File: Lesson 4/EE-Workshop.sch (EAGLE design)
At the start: 1 part

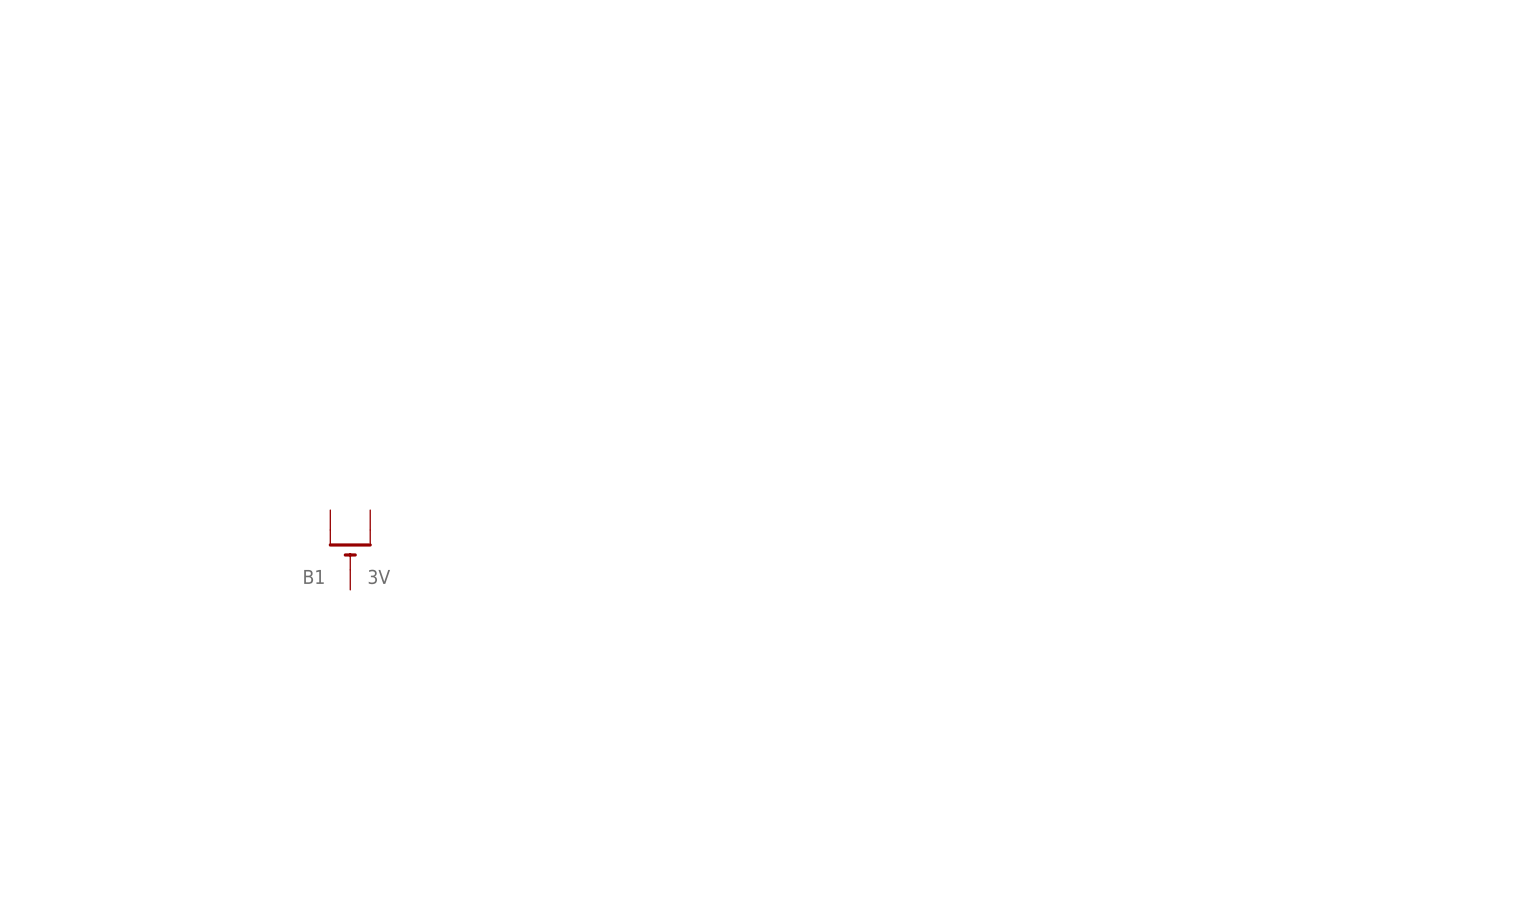
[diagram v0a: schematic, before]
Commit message: Piano
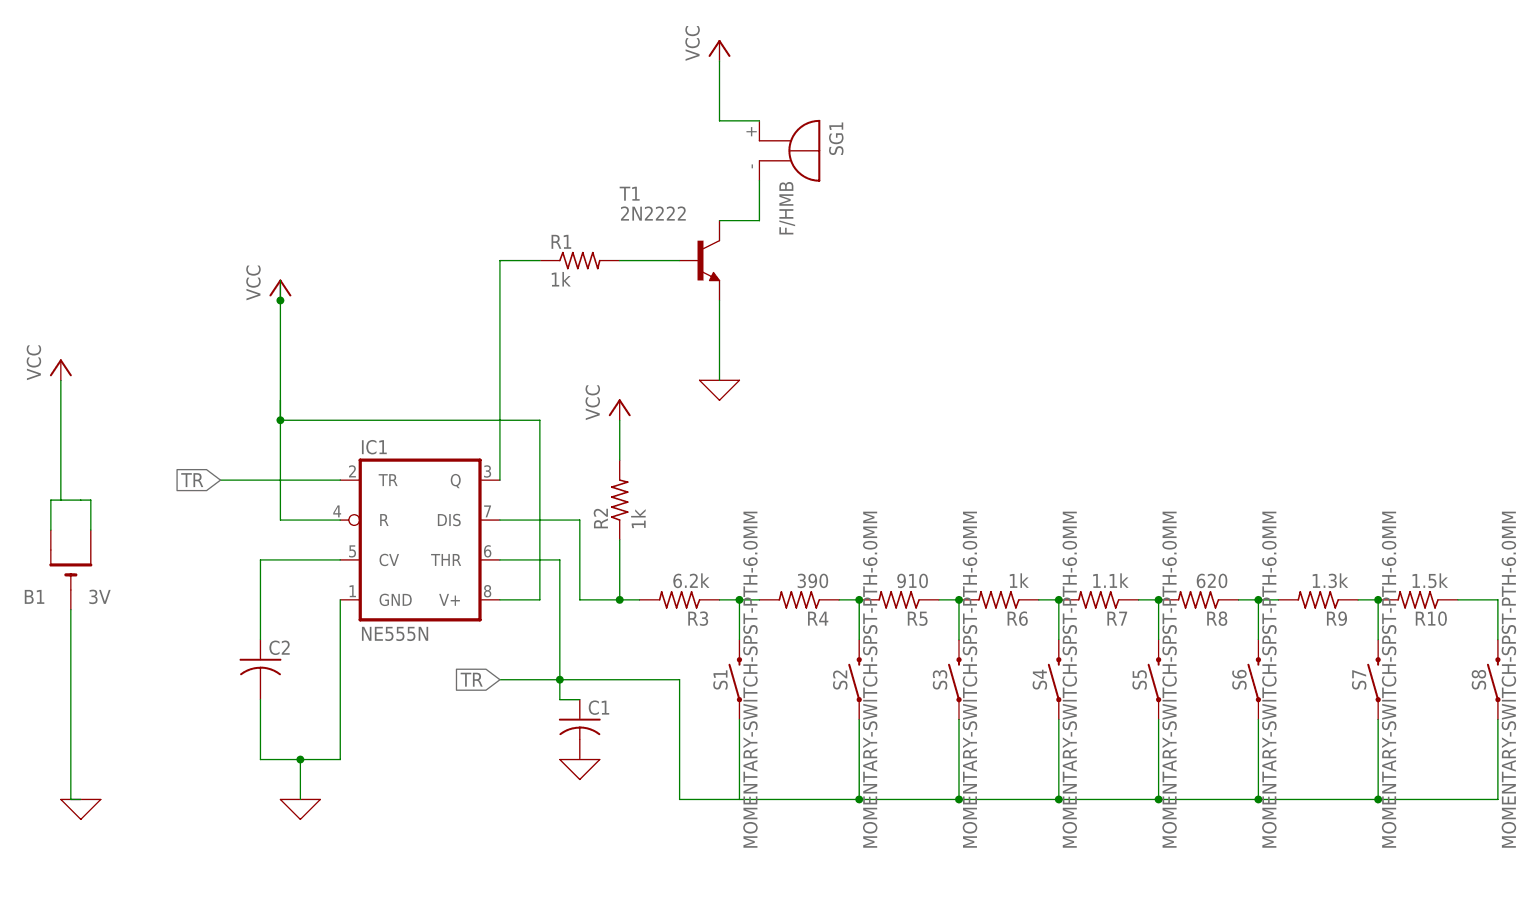
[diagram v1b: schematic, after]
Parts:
- added C1, C2: (no value), rcl:C-US025-025X050
- added IC1: NE555N, linear:NE555N
- added R1, R2, R6: 1k, rcl:R-US_0309/12
- added R10: 1.5k, rcl:R-US_0309/12
- added R3: 6.2k, rcl:R-US_0309/12
- added R4: 390, rcl:R-US_0309/12
- added R5: 910, rcl:R-US_0309/12
- added R7: 1.1k, rcl:R-US_0309/12
- added R8: 620, rcl:R-US_0309/12
- added R9: 1.3k, rcl:R-US_0309/12
- added S1, S2, S3, S4, S5, S6, S7, S8: MOMENTARY-SWITCH-SPST-PTH-6.0MM, SparkFun-Switches:MOMENTARY-SWITCH-SPST-PTH-6.0MM
- added SG1: F/HMB, buzzer:F/HMB
- added T1: 2N2222, transistor:2N2222
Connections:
- new net 0: B1.-, C1.2, C2.2, IC1.GND, T1.E
- new net N$1: C2.1, IC1.CV
- new net N$10: IC1.DIS, R2.1, R3.2
- new net N$11: S1.1, S2.1, S3.1, S4.1, S5.1, S6.1, S7.1, S8.1
- new net N$12: SG1.-, T1.C
- new net N$16: IC1.Q, R1.1
- new net N$17: R1.2, T1.B
- new net N$2: R3.1, R4.2, S1.2
- new net N$3: R4.1, R5.2, S2.2
- new net N$4: R5.1, R6.2, S3.2
- new net N$5: R6.1, R7.2, S4.2
- new net N$6: R7.1, R8.2, S5.2
- new net N$7: R8.1, R9.2, S6.2
- new net N$8: R10.2, R9.1, S7.2
- new net N$9: R10.1, S8.2
- new net TR: C1.1, IC1.THR, IC1.TR
- new net VCC: B1.+, B1.+1, IC1.R, IC1.V+, R2.2, SG1.+
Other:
- moved on the sheet: B1
